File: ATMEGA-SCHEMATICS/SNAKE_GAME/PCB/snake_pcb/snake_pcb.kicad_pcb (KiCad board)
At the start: 4 copper layers, 180 x 120 mm, 132 parts, among them J1 Conn_01x02_Pin, J10 LCD_SCREEN, J11 EXT_ACC_PROG, J12 JUMPER, J13 Conn_01x04_Pin, J14 Conn_01x05_Pin, J15 Conn_01x04_Pin, J16 Conn_01x06_Pin, J17 Conn_01x06_Pin, J18 Conn_01x05_Pin, J19 Conn_01x06_Pin, J2 GRID, J20 Conn_01x06_Pin, J21 Conn_01x04_Pin, J22 Conn_01x06_Pin, J23 Conn_01x06_Pin, J24 Conn_01x05_Pin, J25 Conn_01x02_Pin, J26 B_START, J27 B_STOP, J28 B_SELECT, J3 USB_A, J4 Barrel_Jack_Switch, J5 Conn_01x03_Pin, J6 TERM_GAME, J7 TERM_GRID, J9 Conn_01x05_Pin, SW1 PROG_SWT, SW2 SW_Push, SW3 SW_Push, SW4 SW_Push, SW5 SW_Push, U1 ATmega168A-P, U2 ATmega168A-P, U3 ATmega8A-P, U4 CD4066BE, U5 FT232RL, U6 CD4066BE, U7 CD4066BE, U8 MX25L3233FM1, U9 AMS1117-3.3, Y1 Crystal, Y2 Crystal, Y3 Crystal

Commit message: .
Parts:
- added 47uF1: C_Polarized, Capacitor_THT:C_Disc_D3.0mm_W1.6mm_P2.50mm, F.Cu at (220.5, 87.8)
- added 47uF2: C_Polarized, Capacitor_THT:C_Disc_D3.0mm_W1.6mm_P2.50mm, F.Cu at (255.1, 88.0)
- added 47uF3: C_Polarized, Capacitor_THT:C_Disc_D3.0mm_W1.6mm_P2.50mm, F.Cu at (283.5, 84.8)
- added C44: 1uF, Capacitor_THT:C_Disc_D7.5mm_W5.0mm_P5.00mm, F.Cu at (267.5, 96.5)
- added C46: 1uF, Capacitor_THT:C_Disc_D7.5mm_W5.0mm_P5.00mm, F.Cu at (236.1, 100.0)
- added C77: 1uF, Capacitor_THT:C_Disc_D7.5mm_W5.0mm_P5.00mm, F.Cu at (203.0, 95.5)
- added D4: V_METER- LED, LED_THT:LED_D1.8mm_W3.3mm_H2.4mm, F.Cu at (249.1, 88.3)
- added D5: V_METER- LED, LED_THT:LED_D1.8mm_W3.3mm_H2.4mm, F.Cu at (278.0, 85.0)
- added D6: 1N914, Diode_THT:D_DO-35_SOD27_P7.62mm_Horizontal, F.Cu at (222.0, 99.3)
- added D7: V_METER- LED, LED_THT:LED_D1.8mm_W3.3mm_H2.4mm, F.Cu at (214.5, 85.2)
- added D8: 1N914, Diode_THT:D_DO-35_SOD27_P7.62mm_Horizontal, F.Cu at (255.1, 102.9)
- added D9: 1N914, Diode_THT:D_DO-35_SOD27_P7.62mm_Horizontal, F.Cu at (287.0, 100.8)
- added R28: 4.7k, Resistor_THT:R_Axial_DIN0207_L6.3mm_D2.5mm_P10.16mm_Horizontal, F.Cu at (210.6, 87.5)
- added R30: 4.7k, Resistor_THT:R_Axial_DIN0207_L6.3mm_D2.5mm_P10.16mm_Horizontal, F.Cu at (281.5, 110.0)
- added R36: 1k, Resistor_THT:R_Axial_DIN0207_L6.3mm_D2.5mm_P10.16mm_Horizontal, F.Cu at (244.7, 86.0)
- added R37: 4.7k, Resistor_THT:R_Axial_DIN0207_L6.3mm_D2.5mm_P10.16mm_Horizontal, F.Cu at (273.6, 87.5)
- added R38: 4.7k, Resistor_THT:R_Axial_DIN0207_L6.3mm_D2.5mm_P10.16mm_Horizontal, F.Cu at (249.6, 112.6)
- added R39: 1k, Resistor_THT:R_Axial_DIN0207_L6.3mm_D2.5mm_P10.16mm_Horizontal, F.Cu at (273.6, 83.5)
- added R54: 1k, Resistor_THT:R_Axial_DIN0207_L6.3mm_D2.5mm_P10.16mm_Horizontal, F.Cu at (210.6, 83.5)
- added R56: 4.7k, Resistor_THT:R_Axial_DIN0207_L6.3mm_D2.5mm_P10.16mm_Horizontal, F.Cu at (217.0, 109.6)
- added R57: 4.7k, Resistor_THT:R_Axial_DIN0207_L6.3mm_D2.5mm_P10.16mm_Horizontal, F.Cu at (244.7, 90.5)
- added TPS75533KCG1: ~, Package_TO_SOT_THT:TO-220-5_Vertical, F.Cu at (210.1, 96.0)
- added TPS75533KCG2: ~, Package_TO_SOT_THT:TO-220-5_Vertical, F.Cu at (242.7, 98.5)
- added TPS75533KCG3: ~, Package_TO_SOT_THT:TO-220-5_Vertical, F.Cu at (273.9, 95.5)
- moved C1 101.8 mm to (192.4, 213.0)
- moved C11 101.8 mm to (241.1, 185.1)
- moved C24 101.8 mm to (268.0, 149.5)
- moved C25 101.8 mm to (237.5, 141.6)
- moved C27 101.8 mm to (270.3, 143.8)
- moved C28 101.8 mm to (270.3, 136.8)
- moved C3 101.8 mm to (192.4, 220.0)
- moved C30 101.8 mm to (223.0, 120.4)
- moved C31 101.8 mm to (293.8, 116.5)
- moved C4 101.8 mm to (225.4, 212.5)
- moved C40 101.8 mm to (282.8, 116.5)
- moved C5 101.8 mm to (223.9, 217.5)
- moved J13 101.8 mm to (261.3, 137.1)
- moved J2 101.8 mm to (291.8, 157.4)
- moved J20 101.8 mm to (241.3, 162.5)
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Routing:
- net /game/B_SELECT: track 85.3 -> 22.9 mm
- net /game/SDA_GAME: track 36.2 -> 11.1 mm
- net /game/RESET_GAME: track 5.91 -> 18.9 mm
- net /game/FLASH_CS: track 0.00 -> 11.1 mm
- net /game/PB2: track 0.00 -> 10.6 mm
- net /game/SCK_GAME: track 0.00 -> 6.12 mm
- net /game/MISO_GAME: track 0.00 -> 6.12 mm
- net /game/MOSI_GAME: track 0.00 -> 6.12 mm
- removed copper zone on F.Cu, net (none)
- removed copper zone on In1.Cu, net (none)
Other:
- board size 180 x 120 mm -> 200 x 200 mm

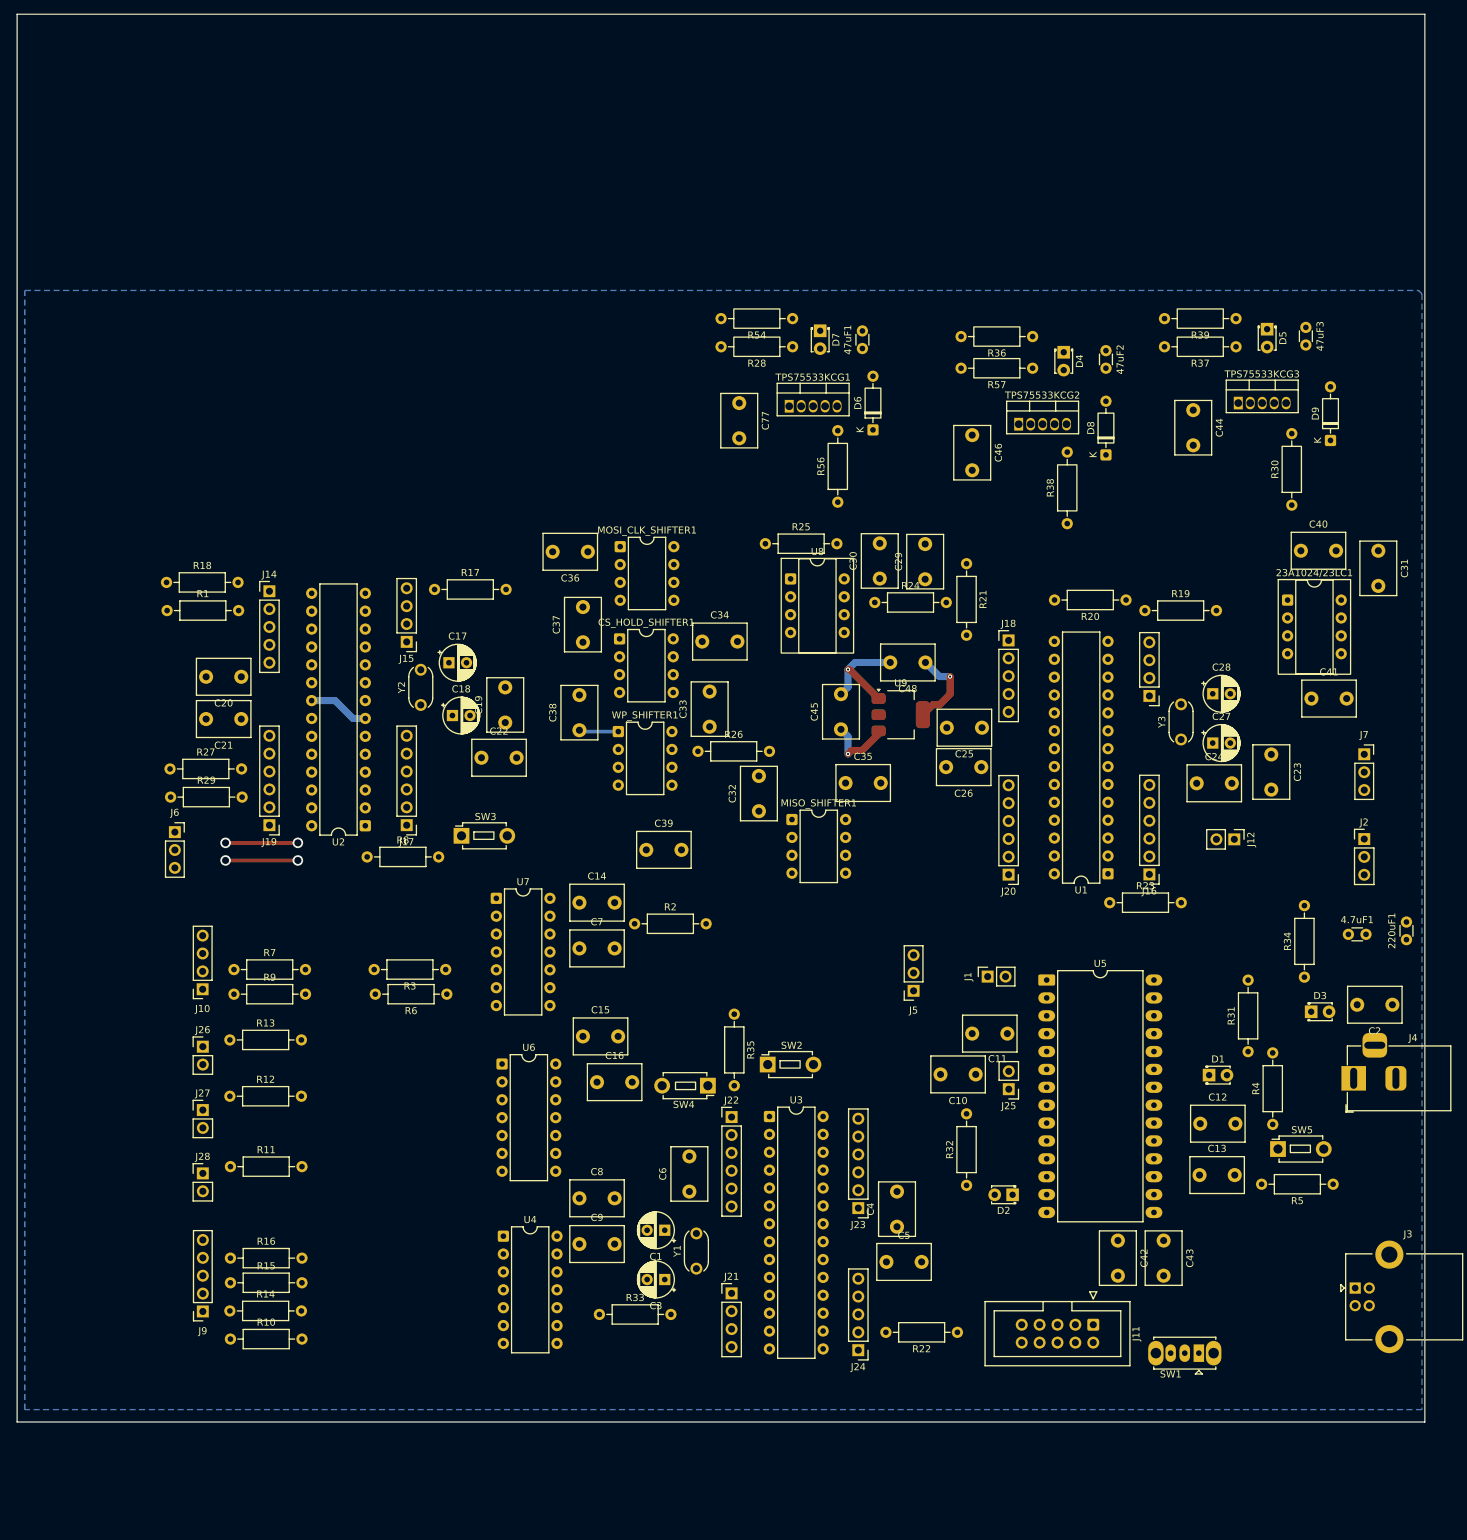
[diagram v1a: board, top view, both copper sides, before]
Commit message: ...
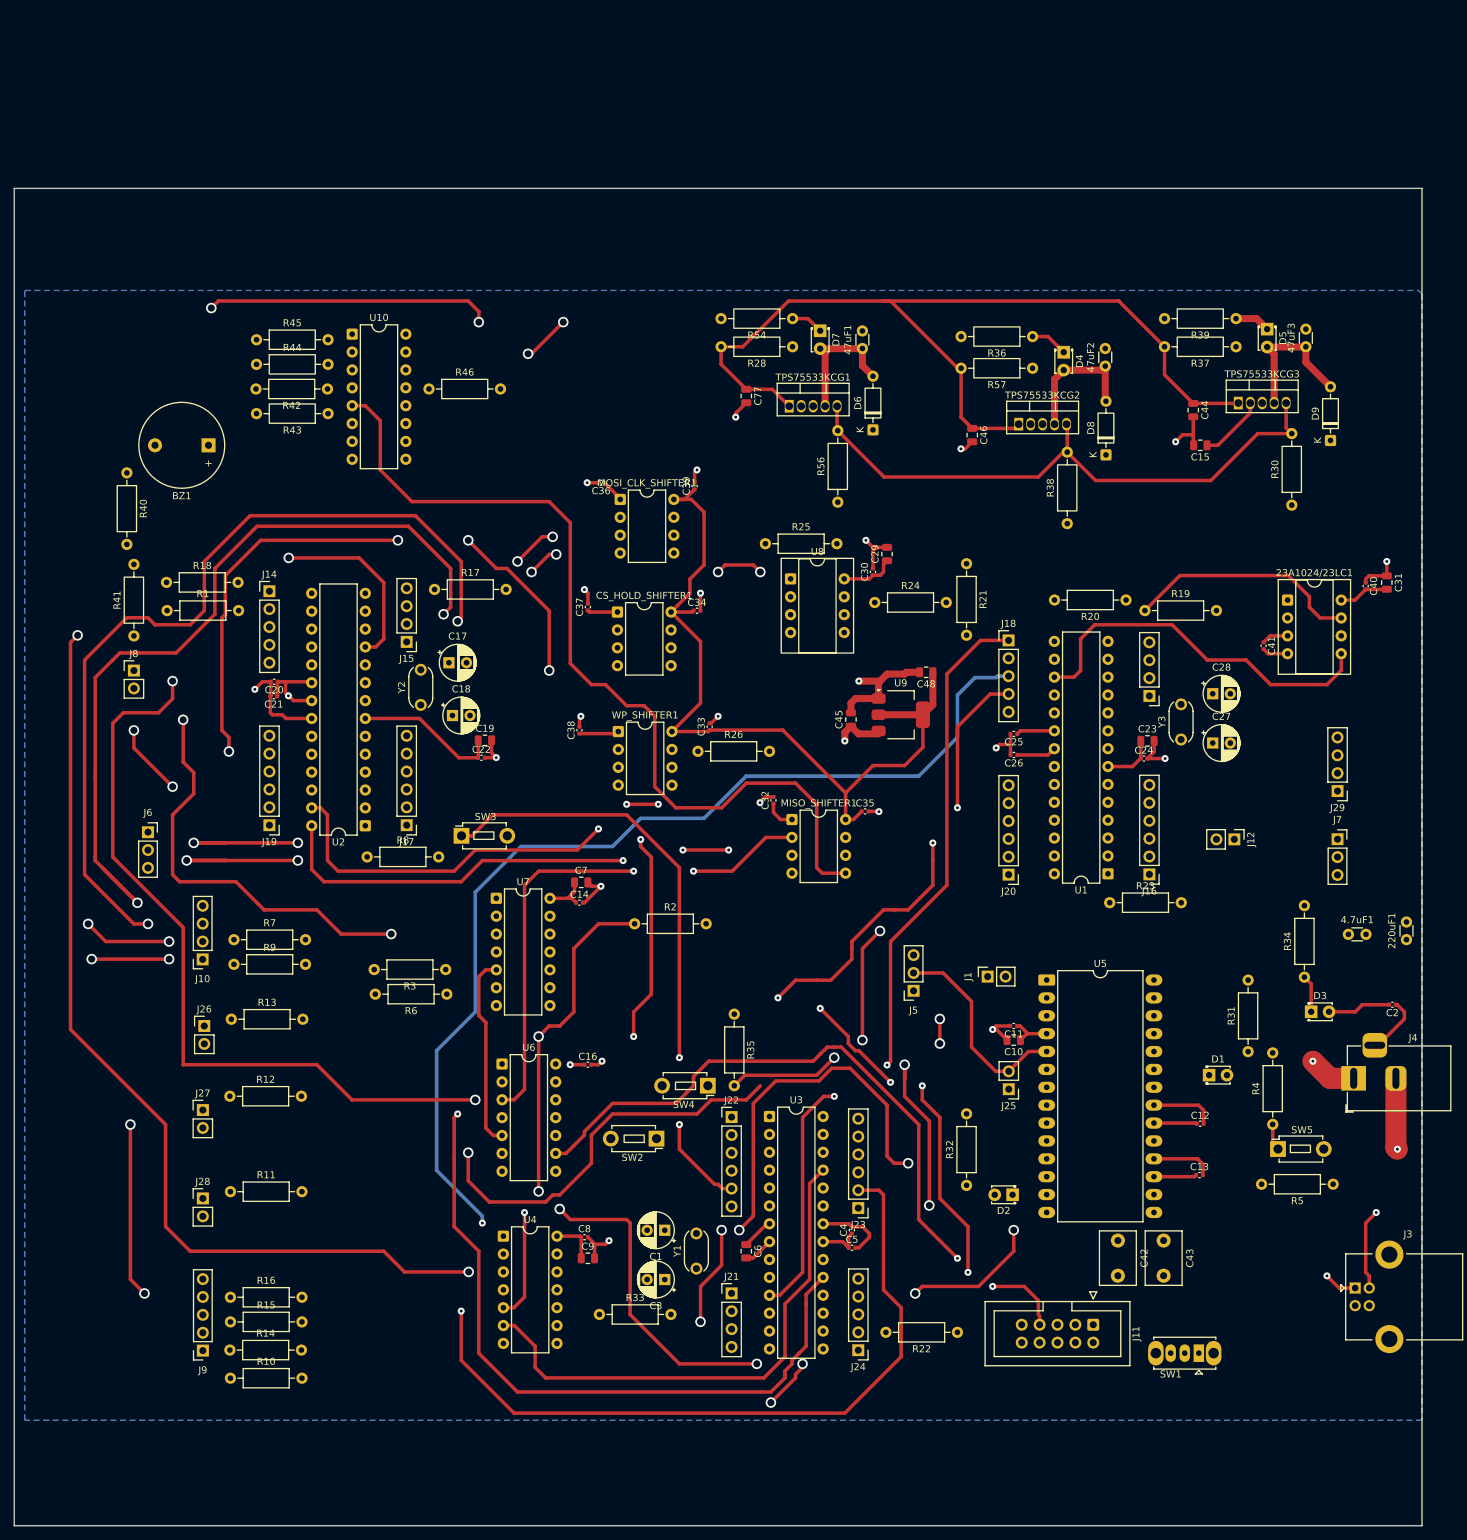
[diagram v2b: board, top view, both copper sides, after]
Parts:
- removed J2: GRID, Connector_PinHeader_2.54mm:PinHeader_1x03_P2.54mm_Vertical
- removed R27, R29: 10K, Resistor_THT:R_Axial_DIN0207_L6.3mm_D2.5mm_P10.16mm_Horizontal
- added BZ1: Buzzer, Buzzer_Beeper:Buzzer_12x9.5RM7.6, F.Cu at (127.6, 101.5)
- added J29: GRID, Connector_PinHeader_2.54mm:PinHeader_1x04_P2.54mm_Vertical, F.Cu at (288.0, 150.6)
- added J8: Vibrator, Connector_PinHeader_2.54mm:PinHeader_1x02_P2.54mm_Vertical, F.Cu at (117.0, 133.5)
- added R40: 200, Resistor_THT:R_Axial_DIN0207_L6.3mm_D2.5mm_P10.16mm_Horizontal, F.Cu at (116.0, 105.4)
- added R41: 200, Resistor_THT:R_Axial_DIN0207_L6.3mm_D2.5mm_P10.16mm_Horizontal, F.Cu at (117.0, 128.6)
- added R42: 10K, Resistor_THT:R_Axial_DIN0207_L6.3mm_D2.5mm_P10.16mm_Horizontal, F.Cu at (144.5, 93.5)
- added R43: 10K, Resistor_THT:R_Axial_DIN0207_L6.3mm_D2.5mm_P10.16mm_Horizontal, F.Cu at (144.6, 97.0)
- added R44: 10K, Resistor_THT:R_Axial_DIN0207_L6.3mm_D2.5mm_P10.16mm_Horizontal, F.Cu at (134.4, 90.0)
- added R45: 10K, Resistor_THT:R_Axial_DIN0207_L6.3mm_D2.5mm_P10.16mm_Horizontal, F.Cu at (134.4, 86.5)
- added R46: 10K, Resistor_THT:R_Axial_DIN0207_L6.3mm_D2.5mm_P10.16mm_Horizontal, F.Cu at (158.9, 93.5)
- added U10: PCF8574AP, Package_DIP:DIP-16_W7.62mm, F.Cu at (148.0, 85.7)
- C10, C15, C19, C23, C29, C31, C44, C45, C46, C48, C6, C7, C77, C9: footprint Capacitor_THT:C_Disc_D7.5mm_W5.0mm_P5.00mm -> Capacitor_SMD:C_0805_2012Metric
- C11, C12, C13, C14, C16, C2, C20, C21, C22, C24, C25, C26, C30, C32, C33, C34, C35, C36, C37, C38, C39, C4, C40, C41, C5, C8: footprint Capacitor_THT:C_Disc_D7.5mm_W5.0mm_P5.00mm -> Capacitor_SMD:C_0402_1005Metric
- moved C15 121.4 mm to (268.5, 101.5), turned to 180 degrees
- moved C39 52.2 mm to (196.7, 107.3), turned to 90 degrees
- moved SW2 19.0 mm to (191.2, 200.0), turned to 180 degrees
- moved C23 17.7 mm to (261.0, 143.5), turned to 0 degrees
- moved J7 12.6 mm to (288.0, 157.5)
- moved C6 11.7 mm to (204.0, 216.0), turned to -90 degrees
- moved C40 10.5 mm to (292.0, 121.5), turned to -90 degrees
- moved C41 10.1 mm to (277.5, 130.0), turned to -90 degrees
- moved C36 9.99 mm to (183.4, 106.8)
- moved C7 9.38 mm to (180.6, 163.6)
- moved C24 8.28 mm to (260.5, 146.0)
- moved C10 7.28 mm to (242.0, 186.0)
- moved MOSI_CLK_SHIFTER1 6.71 mm to (186.1, 109.2)
- moved C29 6.49 mm to (224.0, 117.0)
- moved C4 6.43 mm to (219.0, 213.0)
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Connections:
- CS_HOLD_SHIFTER1 pad 5: /game/PC2 -> /game/DIR_MCU_T_FLASH
- J15 pad 1: /game/J_RIGHT -> /game/BUZZER_PWM
- J19 pad 3: /game/PC3 -> /game/VIBRATOR
- J19 pad 4: /game/PC2 -> /game/J_RIGHT
- MISO_SHIFTER1 pad 5: /game/PC3 -> /game/DIR_FLASH_T_MCU
- MOSI_CLK_SHIFTER1 pad 5: /game/PC2 -> /game/DIR_MCU_T_FLASH
- U2 pad 11: /game/J_RIGHT -> /game/BUZZER_PWM
- U2 pad 25: /game/PC2 -> /game/J_RIGHT
- U2 pad 26: /game/PC3 -> /game/VIBRATOR
- WP_SHIFTER1 pad 5: /game/PC2 -> /game/DIR_MCU_T_FLASH
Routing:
- net /game/SCL_GAME: track 32.3 -> 355.6 mm, vias 0 -> 5
- net /game/SDA_GAME: track 11.1 -> 329.9 mm, vias 0 -> 7
- net /programmer/EXT_SIGNAL: track 0.00 -> 267.5 mm, vias 0 -> 1
- net /game/MOSI_GAME: track 6.12 -> 233.3 mm, vias 0 -> 4
- net /grid/MOSI_GRID: track 0.00 -> 210.3 mm, vias 0 -> 1
- net /game/MISO_GAME: track 6.12 -> 209.6 mm, vias 0 -> 4
- net /game/FLASH_CS: track 11.1 -> 191.5 mm, vias 0 -> 4
- net /grid/SCK_GRID: track 0.00 -> 179.5 mm, vias 0 -> 2
- net /programmer/GAME_SIGNAL: track 0.00 -> 178.8 mm, vias 0 -> 2
- net /programmer/GRID_SIGNAL: track 0.00 -> 178.5 mm, vias 0 -> 2
- net /grid/MISO_GRID: track 0.00 -> 173.6 mm, vias 0 -> 3
- net /grid/SRAM_CS: track 0.00 -> 170.8 mm, vias 0 -> 2
- net /game/B_STOP: track 4.65 -> 167.4 mm, vias 0 -> 2
- net /game/B_START: track 4.24 -> 158.3 mm, vias 0 -> 2
- net GND: track 16.4 -> 169.7 mm, vias 1 -> 24
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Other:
- board size 200 x 200 mm -> 200 x 190 mm
